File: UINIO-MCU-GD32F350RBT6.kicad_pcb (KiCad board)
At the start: 2 copper layers, 81.5 x 20.3 mm, 39 parts, among them J1 Conn_01x32_Male, J2 Conn_01x32_Male, J3 Conn_01x04_Male, SW1 BOOT0, SW2 NRST, U1 ME6211C33M5G-N, U2 GD32F350RBT6, Y1 32.768KHz, Y2 8MHz

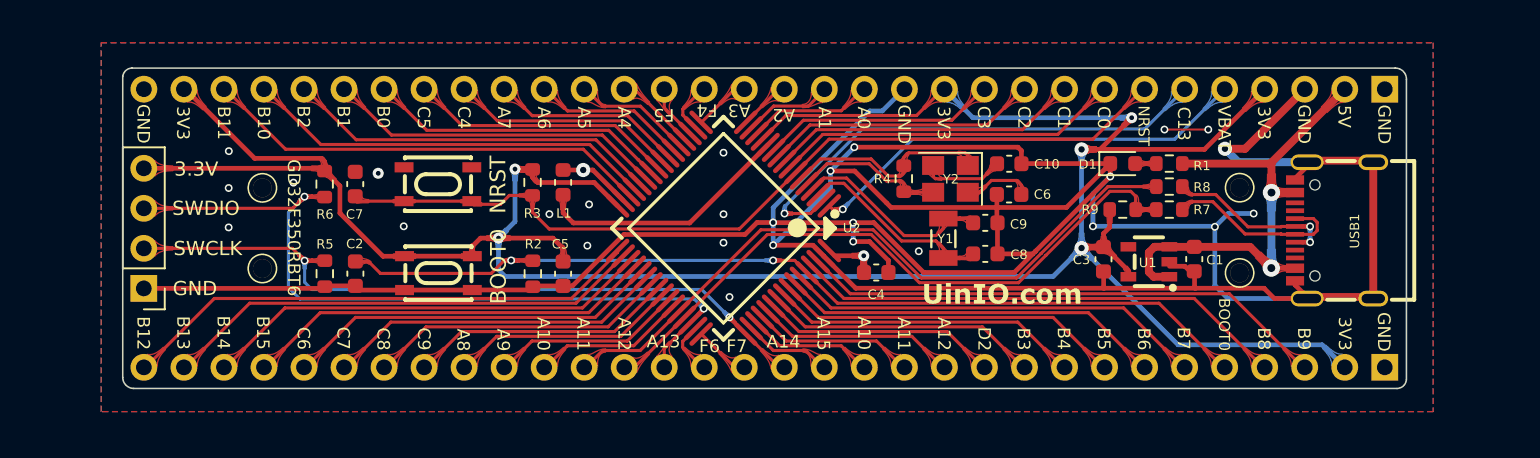
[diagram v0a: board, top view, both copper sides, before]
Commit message: Upgrade version 2.0.0.
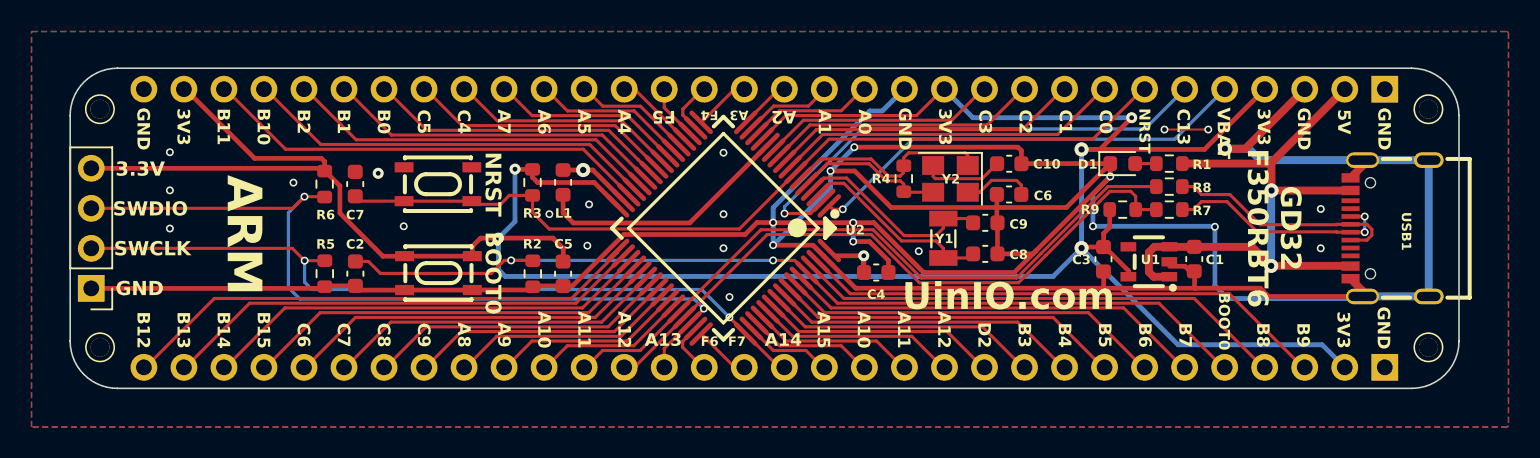
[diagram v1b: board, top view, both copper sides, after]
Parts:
- removed the ? at (167.3, 107.8)
- removed the ? at (173.3, 103.8)
- removed the ? at (142.8, 103.5)
- removed the ? at (167.5, 103.8)
- added ?: LOGO, LOGO, B.Cu at (171.6, 103.6)
- added ?: LOGO, LOGO, B.Cu at (137.2, 103.6)
- J1, J2: value Conn_01x32_Male -> Conn_01x32_Pin
- J3: value Conn_01x04_Male -> Conn_01x04_Pin
- moved HOLE3 13.0 mm to (194.3, 96.1)
- moved HOLE4 12.9 mm to (194.3, 111.2)
- moved HOLE1 11.5 mm to (110.0, 96.1)
- moved HOLE2 11.4 mm to (110.1, 111.2)
- moved USB1 3.52 mm to (191.9, 103.6)
- moved J3 3.33 mm to (109.5, 107.4)
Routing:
- net GND: track 239.4 -> 250.8 mm, vias 28 -> 29
- net /VDD_5V: track 33.1 -> 40.0 mm
- net /USB_Data-: track 11.1 -> 15.0 mm, vias 2 -> 0
- net /PA14/SWCLK: track 45.6 -> 49.0 mm
- net /PA13/SWDIO: track 49.7 -> 53.1 mm
- net /VDD_3.3V: track 181.4 -> 184.7 mm
- net /USB_Data+: track 11.7 -> 14.5 mm, vias 0 -> 2
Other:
- board size 81.5 x 20.3 mm -> 88.1 x 20.3 mm
- board text added: "ARM"
- board text added: "GD32 F350RBT6"
- board text added: "UinIO.com"
- board text added: "Version 2.0.0"
- board text removed: "GD32F350RBT6"
- board text removed: "Version 1.0.0"
